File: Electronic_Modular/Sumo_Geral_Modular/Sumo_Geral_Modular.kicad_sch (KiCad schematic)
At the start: 26 parts, among them J1 Conn_01x02, J10 Conn_01x03, J11 Conn_01x03, J2 Conn_01x05, J3 Conn_01x05, J4 Conn_01x05, J5 Conn_01x03, J6 Conn_01x08, J7 Conn_01x08, J8 Conn_01x02, J9 Conn_01x02, SW1 SW_Push, SW2 SW_Push, SW3 SW_Push, U1 AMS1117-5.0, U2 AMS1117-3.3

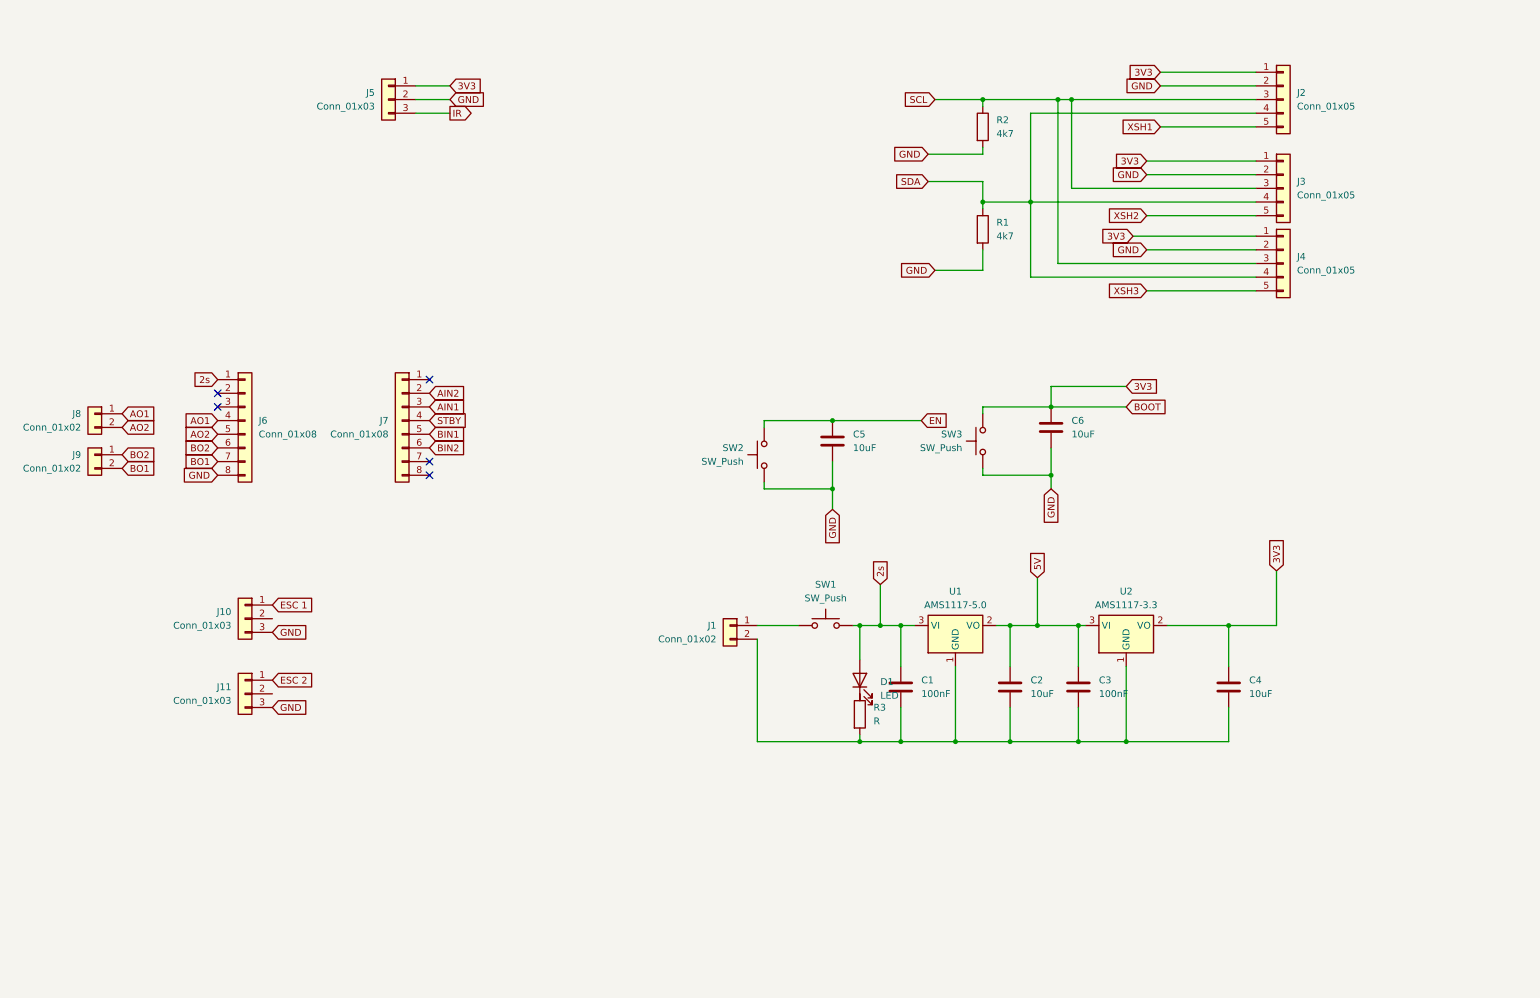
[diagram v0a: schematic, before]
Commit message: chore: continue development modular pcb
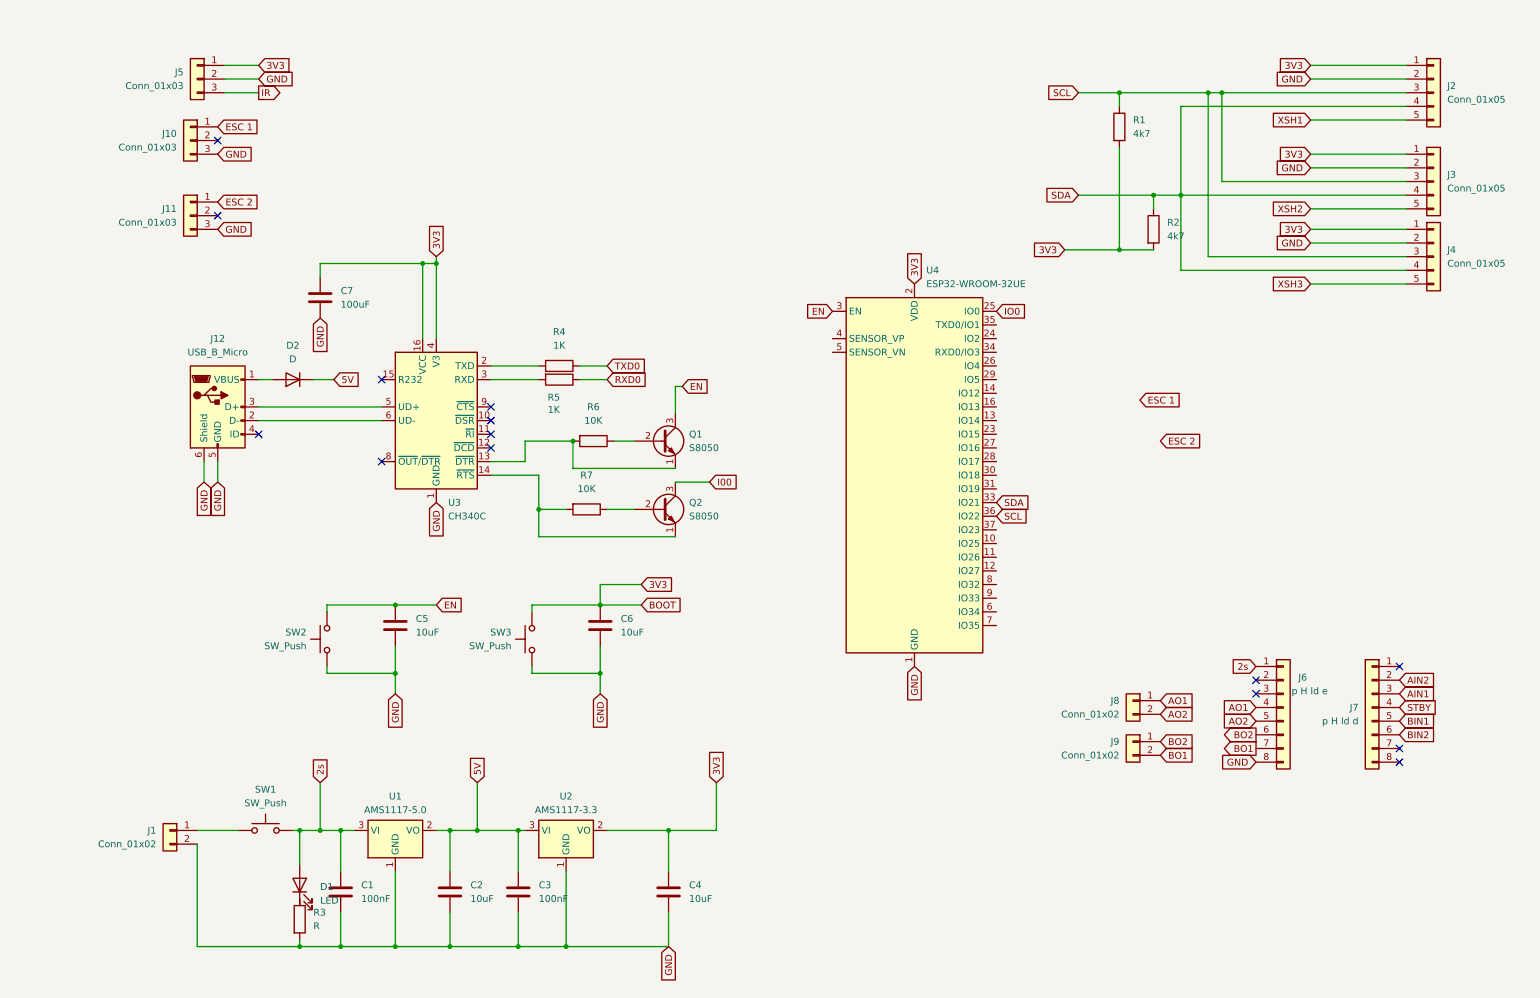
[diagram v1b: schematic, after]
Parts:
- added C7: 100uF, symbol Device:C
- added D2: D, symbol Device:D
- added J12: USB_B_Micro, symbol Connector:USB_B_Micro
- added Q1, Q2: S8050, Package_TO_SOT_THT:TO-92_Inline, symbol Transistor_BJT:S8050
- added R4, R5: 1K, symbol Device:R
- added R6, R7: 10K, symbol Device:R
- added U3: CH340C, Package_SO:SOIC-16_3.9x9.9mm_P1.27mm, symbol Interface_USB:CH340C
- added U4: ESP32-WROOM-32UE, RF_Module:ESP32-WROOM-32UE, symbol RF_Module:ESP32-WROOM-32UE
- J6: value Conn_01x08 -> p H ld e
- J7: value Conn_01x08 -> p H ld d
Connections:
- net 3V3: now also R1.2, R2.2, C7.1, U3.16 (VCC), U3.4 (V3), U4.2 (VDD)
- net 5V: now also D2.1 (K)
- net EN: now also Q1.3 (C), U4.3 (EN)
- net GND: now also C1.2, C2.2, C3.2, C4.2, J1.2 (Pin_2), R3.2, U1.1 (GND), U2.1 (GND), C7.2, J12.5 (GND), J12.6 (Shield), U3.1 (GND), U4.1 (GND), U4.15 (GND), U4.38 (GND), U4.39 (GND); no longer R1.2, R2.2
- net SCL: now also R1.1, U4.36 (IO22); no longer R2.1
- net SDA: now also R2.1, U4.33 (IO21); no longer R1.1
- new net: R5.2, U3.3 (RXD)
- new net: Q2.1 (E), R7.2, U3.14 (~{RTS})
- new net: Q2.2 (B), R7.1
- new net: D2.2 (A), J12.1 (VBUS)
- new net: J12.2 (D-), U3.6 (UD-)
- new net: J12.3 (D+), U3.5 (UD+)
- new net: Q1.1 (E), R6.2, U3.13 (~{DTR})
- new net: Q1.2 (B), R6.1
- new net: R4.2, U3.2 (TXD)
- new net I00: Q2.3 (C)
- new net IO0: U4.25 (IO0)
- new net RXD0: R5.1
- new net TXD0: R4.1
- no-connect marks 5 -> 14
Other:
- moved on the sheet: C1, C2, C3, C4, C5, C6, D1, J1, J10, J11, J2, J3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

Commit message: chore: finish the schematic and set footprints
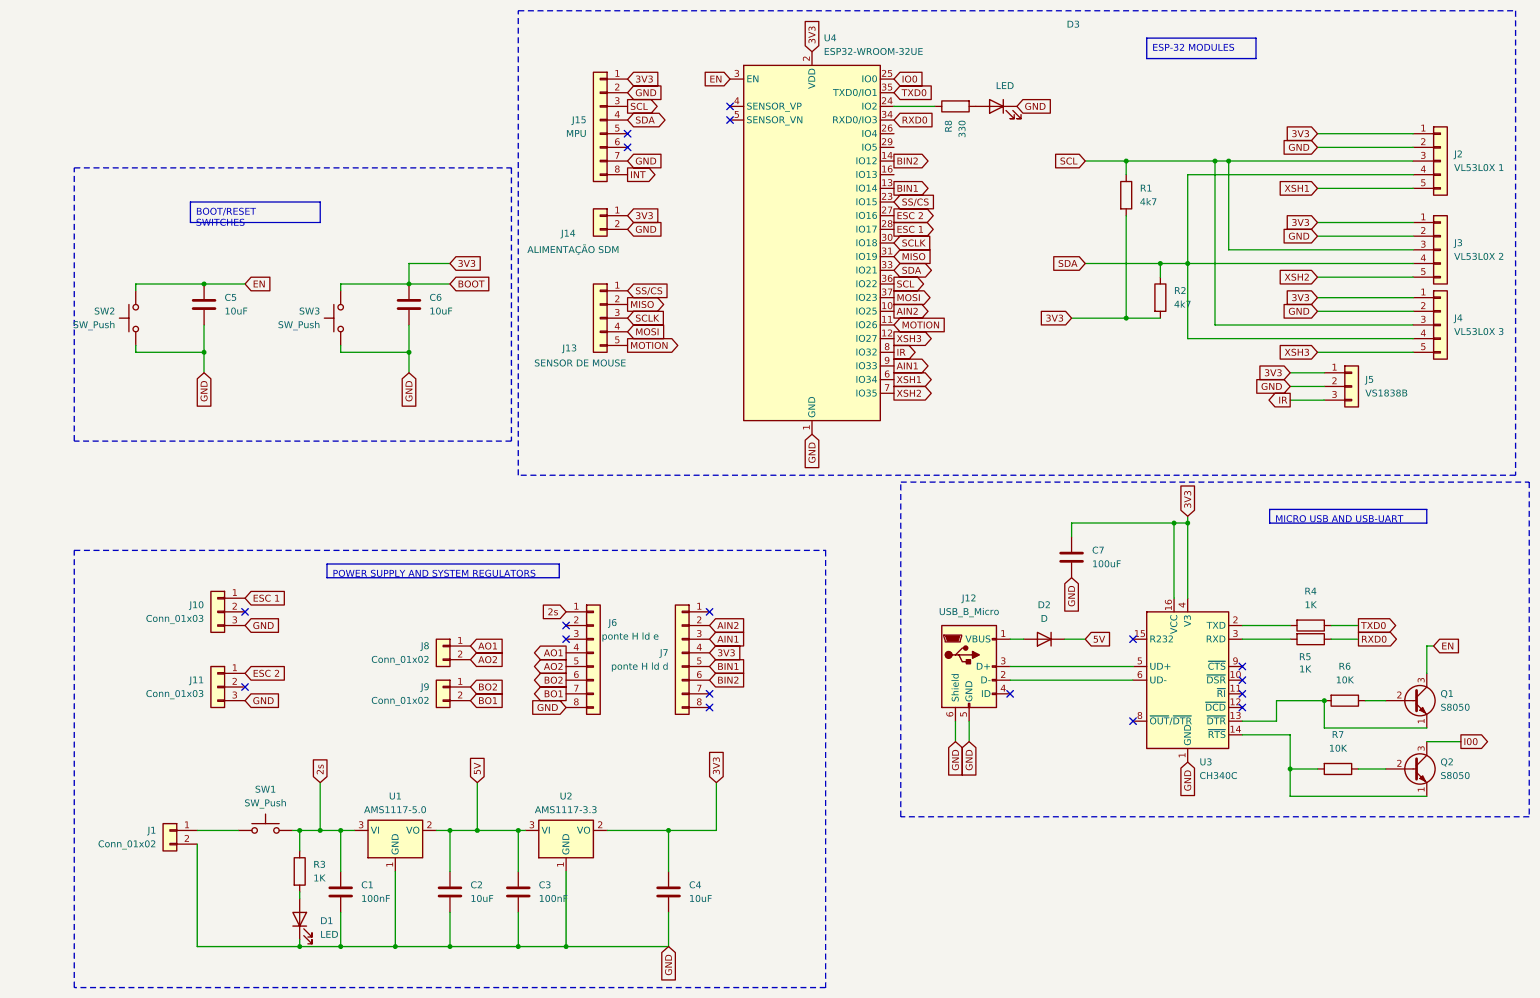
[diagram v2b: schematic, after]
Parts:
- added D3: LED, symbol Device:LED
- added J13: SENSOR DE MOUSE, Connector_JST:JST_XH_S5B-XH-A_1x05_P2.50mm_Horizontal, symbol Connector_Generic:Conn_01x05
- added J14: ALIMENTAÇÃO SDM, Connector_JST:JST_XH_S2B-XH-A_1x02_P2.50mm_Horizontal, symbol Connector_Generic:Conn_01x02
- added J15: MPU, Connector_PinSocket_2.54mm:PinSocket_1x08_P2.54mm_Vertical, symbol Connector_Generic:Conn_01x08
- added R8: 330, symbol Device:R
- J2: value Conn_01x05 -> VL53L0X 1; footprint (none) -> Connector_JST:JST_XH_B5B-XH-AM_1x05_P2.50mm_Vertical
- J3: value Conn_01x05 -> VL53L0X 2; footprint (none) -> Connector_JST:JST_XH_B5B-XH-AM_1x05_P2.50mm_Vertical
- J4: value Conn_01x05 -> VL53L0X 3; footprint (none) -> Connector_JST:JST_XH_B5B-XH-AM_1x05_P2.50mm_Vertical
- J5: value Conn_01x03 -> VS1838B; footprint (none) -> Connector_PinHeader_2.54mm:PinHeader_1x03_P2.54mm_Vertical
- J6: value p H ld e -> ponte H ld e; footprint (none) -> Connector_PinSocket_2.54mm:PinSocket_1x08_P2.54mm_Vertical
- J7: value p H ld d -> ponte H ld d; footprint (none) -> Connector_PinSocket_2.54mm:PinSocket_1x08_P2.54mm_Vertical
- J8, J9: footprint (none) -> Connector_PinSocket_2.54mm:PinSocket_1x02_P2.54mm_Vertical
- R3: value R -> 1K
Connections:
- net STBY is gone; now on net 3V3: J7.4 (Pin_4)
- net 2s: now also R3.1; no longer D1.2 (A)
- net 3V3: now also J14.1 (Pin_1), J15.1 (Pin_1)
- net AIN1: now also U4.9 (IO33)
- net AIN2: now also U4.10 (IO25)
- net BIN1: now also U4.13 (IO14)
- net BIN2: now also U4.14 (IO12)
- net ESC 1: now also U4.28 (IO17)
- net ESC 2: now also U4.27 (IO16)
- net GND: now also D1.1 (K), D3.1 (K), J14.2 (Pin_2), J15.2 (Pin_2), J15.7 (Pin_7); no longer R3.2
- net IR: now also U4.8 (IO32)
- net RXD0: now also U4.34 (RXD0/IO3)
- net SCL: now also J15.3 (Pin_3)
- net SDA: now also J15.4 (Pin_4)
- net TXD0: now also U4.35 (TXD0/IO1)
- net XSH1: now also U4.6 (IO34)
- net XSH2: now also U4.7 (IO35)
- net XSH3: now also U4.12 (IO27)
- net MOTION: now reaches U4.11 (IO26)
- net MOTION: now also J13.5 (Pin_5)
- net SS/CS: now reaches U4.23 (IO15)
- net SS/CS: now also J13.1 (Pin_1)
- net at U4.24 (IO2): now also R8.1
- net SCLK: now reaches U4.30 (IO18)
- net SCLK: now also J13.3 (Pin_3)
- net MISO: now reaches U4.31 (IO19)
- net MISO: now also J13.2 (Pin_2)
- net MOSI: now reaches U4.37 (IO23)
- net MOSI: now also J13.4 (Pin_4)
- new net: D3.2 (A), R8.2
- new net: D1.2 (A), R3.2
- new net INT: J15.8 (Pin_8)
- no-connect marks 14 -> 18
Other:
- moved on the sheet: C5, C6, C7, D1, D2, J10, J11, J12, J2, J3, J4, J5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

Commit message: chore: set all footprints
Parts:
- C1, C2, C3, C4, C5, C6, C7: footprint (none) -> Capacitor_SMD:C_0201_0603Metric
- D1, D3: footprint (none) -> LED_SMD:LED_0201_0603Metric
- D2: footprint (none) -> Diode_SMD:D_0201_0603Metric
- J1: footprint (none) -> Connector_JST:JST_PH_B2B-PH-K_1x02_P2.00mm_Vertical
- J10, J11: footprint (none) -> Connector_JST:JST_XH_B3B-XH-A_1x03_P2.50mm_Vertical
- J12: footprint (none) -> Connector_USB:USB_Micro-B_Amphenol_10118194_Horizontal
- R1, R2, R3, R4, R5, R6, R7, R8: footprint (none) -> Resistor_SMD:R_0201_0603Metric
- SW1: footprint (none) -> Button_Switch_THT:Nidec_Copal_SH-7010C
- SW2, SW3: footprint (none) -> Button_Switch_SMD:SW_SPST_TL3342
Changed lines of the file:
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@@
 			)
 		)
-		(property "Footprint" ""
+		(property "Footprint" "Connector_JST:JST_PH_B2B-PH-K_1x02_P2.00mm_Vertical"
 			(at 30.48 167.64 0)
 			(effects
@@
 			)
 		)
-		(property "Footprint" ""
+		(property "Footprint" "Capacitor_SMD:C_0201_0603Metric"
 			(at 83.5152 182.88 0)
 			(effects
@@
 			)
 		)
-		(property "Footprint" ""
+		(property "Footprint" "Resistor_SMD:R_0201_0603Metric"
 			(at 206.502 49.53 90)
 			(effects
@@
 			)
 		)
-		(property "Footprint" ""
+		(property "Footprint" "Capacitor_SMD:C_0201_0603Metric"
 			(at 124.1552 182.88 0)
 			(effects
@@
 			)
 		)
-		(property "Footprint" ""
+		(property "Footprint" "Resistor_SMD:R_0201_0603Metric"
 			(at 242.57 130.302 90)
 			(effects
@@
 			)
 		)
-		(property "Footprint" ""
+		(property "Footprint" "Capacitor_SMD:C_0201_0603Metric"
 			(at 96.2152 182.88 0)
 			(effects
@@
 			)
 		)
-		(property "Footprint" ""
+		(property "Footprint" "Capacitor_SMD:C_0201_0603Metric"
 			(at 199.0852 120.65 0)
 			(effects
@@
 			)
 		)
-		(property "Footprint" ""
+		(property "Footprint" "Resistor_SMD:R_0201_0603Metric"
 			(at 176.53 31.242 90)
 			(effects
@@
 			)
 		)
-		(property "Footprint" ""
+		(property "Footprint" "Button_Switch_THT:Nidec_Copal_SH-7010C"
 			(at 48.26 162.56 0)
 			(effects
@@
 			)
 		)
-		(property "Footprint" ""
+		(property "Footprint" "Resistor_SMD:R_0201_0603Metric"
 			(at 52.832 175.26 90)
 			(effects
@@
 			)
 		)
-		(property "Footprint" ""
+		(property "Footprint" "Resistor_SMD:R_0201_0603Metric"
 			(at 212.852 68.58 90)
 			(effects
@@
 			)
 		)
-		(property "Footprint" ""
+		(property "Footprint" "LED_SMD:LED_0201_0603Metric"
 			(at 54.61 184.15 0)
 			(effects
@@
 			)
 		)
-		(property "Footprint" ""
+		(property "Footprint" "Connector_USB:USB_Micro-B_Amphenol_10118194_Horizontal"
 			(at 182.88 138.43 0)
 			(effects
@@
 			)
 		)
-		(property "Footprint" ""
+		(property "Footprint" "Connector_JST:JST_XH_B3B-XH-A_1x03_P2.50mm_Vertical"
 			(at 39.37 127 0)
 			(effects
@@
 			)
 		)
-		(property "Footprint" ""
+		(property "Footprint" "Capacitor_SMD:C_0201_0603Metric"
 			(at 75.8952 73.66 0)
 			(effects
@@
 			)
 		)
-		(property "Footprint" ""
+		(property "Footprint" "Resistor_SMD:R_0201_0603Metric"
 			(at 248.92 141.732 90)
 			(effects
@@
 			)
 		)
-		(property "Footprint" ""
+		(property "Footprint" "LED_SMD:LED_0201_0603Metric"
 			(at 184.15 33.02 0)
 			(effects
@@
 			)
 		)
-		(property "Footprint" ""
+		(property "Footprint" "Diode_SMD:D_0201_0603Metric"
 			(at 193.04 132.08 0)
 			(effects
@@
 			)
 		)
-		(property "Footprint" ""
+		(property "Footprint" "Button_Switch_SMD:SW_SPST_TL3342"
 			(at 19.05 72.39 0)
 			(effects
@@
 			)
 		)
-		(property "Footprint" ""
+		(property "Footprint" "Resistor_SMD:R_0201_0603Metric"
 			(at 247.65 154.432 90)
 			(effects
@@
 			)
 		)
-		(property "Footprint" ""
+		(property "Footprint" "Capacitor_SMD:C_0201_0603Metric"
 			(at 63.1952 182.88 0)
 			(effects
@@
 			)
 		)
-		(property "Footprint" ""
+		(property "Footprint" "Button_Switch_SMD:SW_SPST_TL3342"
 			(at 57.15 72.39 0)
 			(effects
@@
 			)
 		)
-		(property "Footprint" ""
+		(property "Footprint" "Capacitor_SMD:C_0201_0603Metric"
 			(at 37.7952 73.66 0)
 			(effects
@@
 			)
 		)
-		(property "Footprint" ""
+		(property "Footprint" "Connector_JST:JST_XH_B3B-XH-A_1x03_P2.50mm_Vertical"
 			(at 39.37 140.97 0)
 			(effects
@@
 			)
 		)
-		(property "Footprint" ""
+		(property "Footprint" "Resistor_SMD:R_0201_0603Metric"
 			(at 242.57 127.762 90)
 			(effects
